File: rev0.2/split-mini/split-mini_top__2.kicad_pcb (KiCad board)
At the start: 2 copper layers, 99.7 x 83.7 mm, 27 parts, among them SW1 SW_PUSH, SW10 SW_PUSH, SW11 SW_PUSH, SW12 SW_PUSH, SW13 SW_PUSH, SW14 SW_PUSH, SW15 SW_PUSH, SW16 SW_PUSH, SW17 SW_PUSH, SW18 SW_PUSH, SW2 SW_PUSH, SW3 SW_PUSH, SW4 SW_PUSH, SW5 SW_PUSH, SW6 SW_PUSH, SW7 SW_PUSH, SW8 SW_PUSH, SW9 SW_PUSH

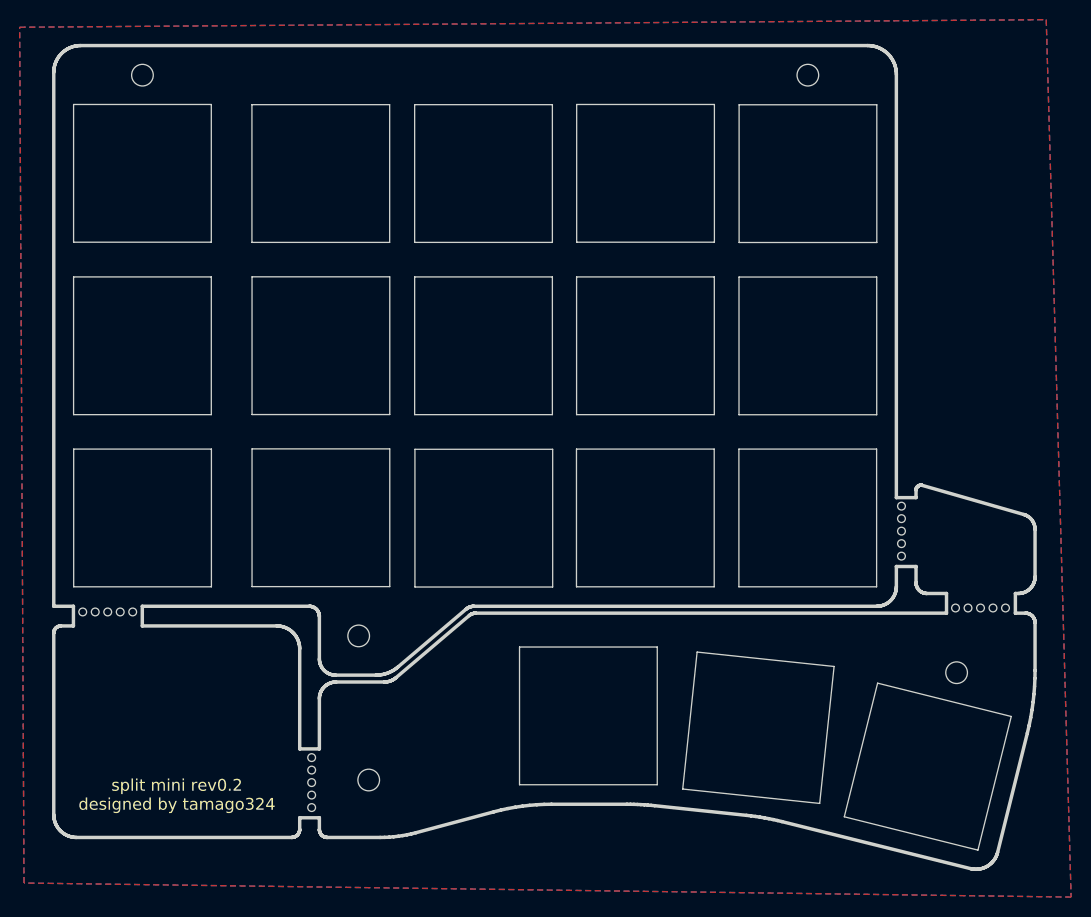
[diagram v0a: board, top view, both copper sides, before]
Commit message: update
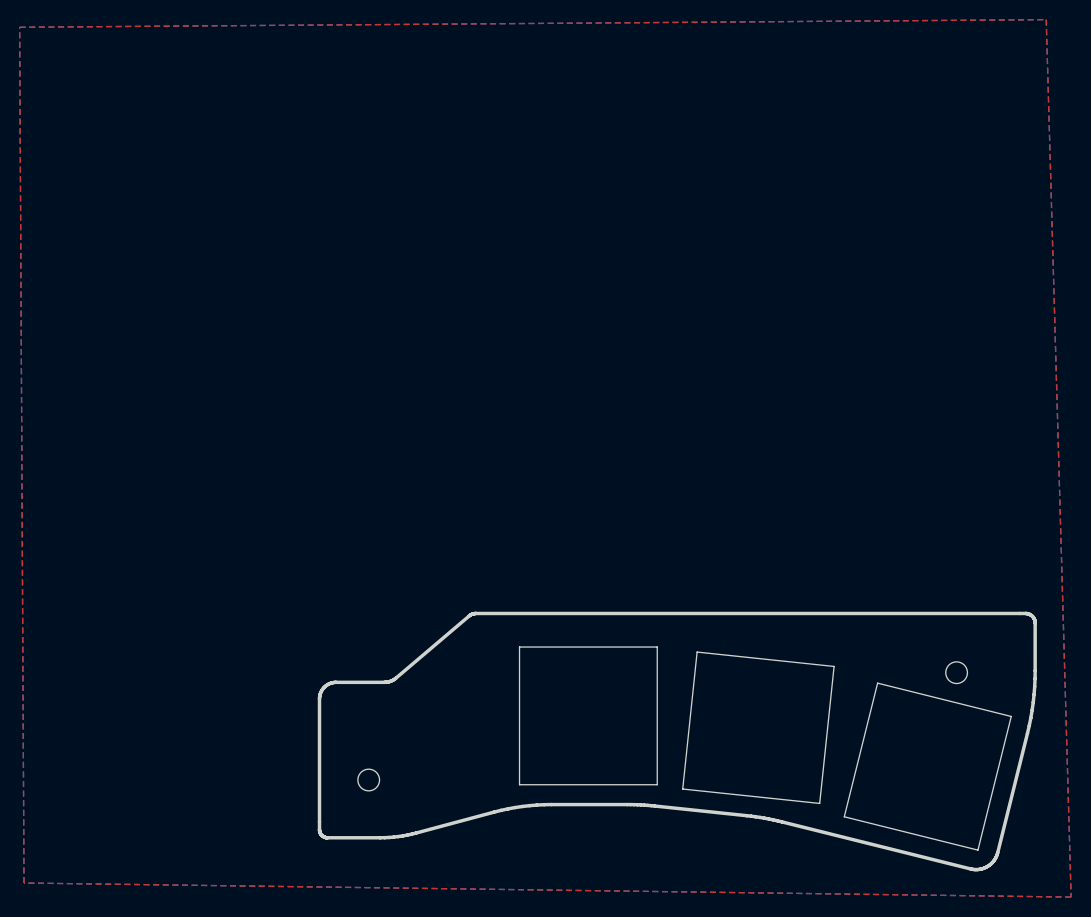
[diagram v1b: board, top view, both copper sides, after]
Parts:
- removed HOLE1, HOLE2, HOLE3: Val**, split-mini:spacer_m2_2.2mm
- removed REF** (x4): breakaway-mousebites, split-mini:breakaway-mousebites
- removed SW1, SW10, SW11, SW12, SW13, SW14, SW15, SW2, SW3, SW4, SW5, SW6, SW7, SW8, SW9: SW_PUSH, split-mini:SW_Hole
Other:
- board size 99.7 x 83.7 mm -> 72.7 x 26 mm
- board text removed: "split mini rev0.2 designed by tamago324"
